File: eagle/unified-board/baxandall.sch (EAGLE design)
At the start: 75 parts, among them IC101 THAT151x, J103 phantom, J104 eqout, J601 micout, U101 OPAMPLME49710, U601 LM3915N, U602 LM3915N, U603 OPAMPLME49710

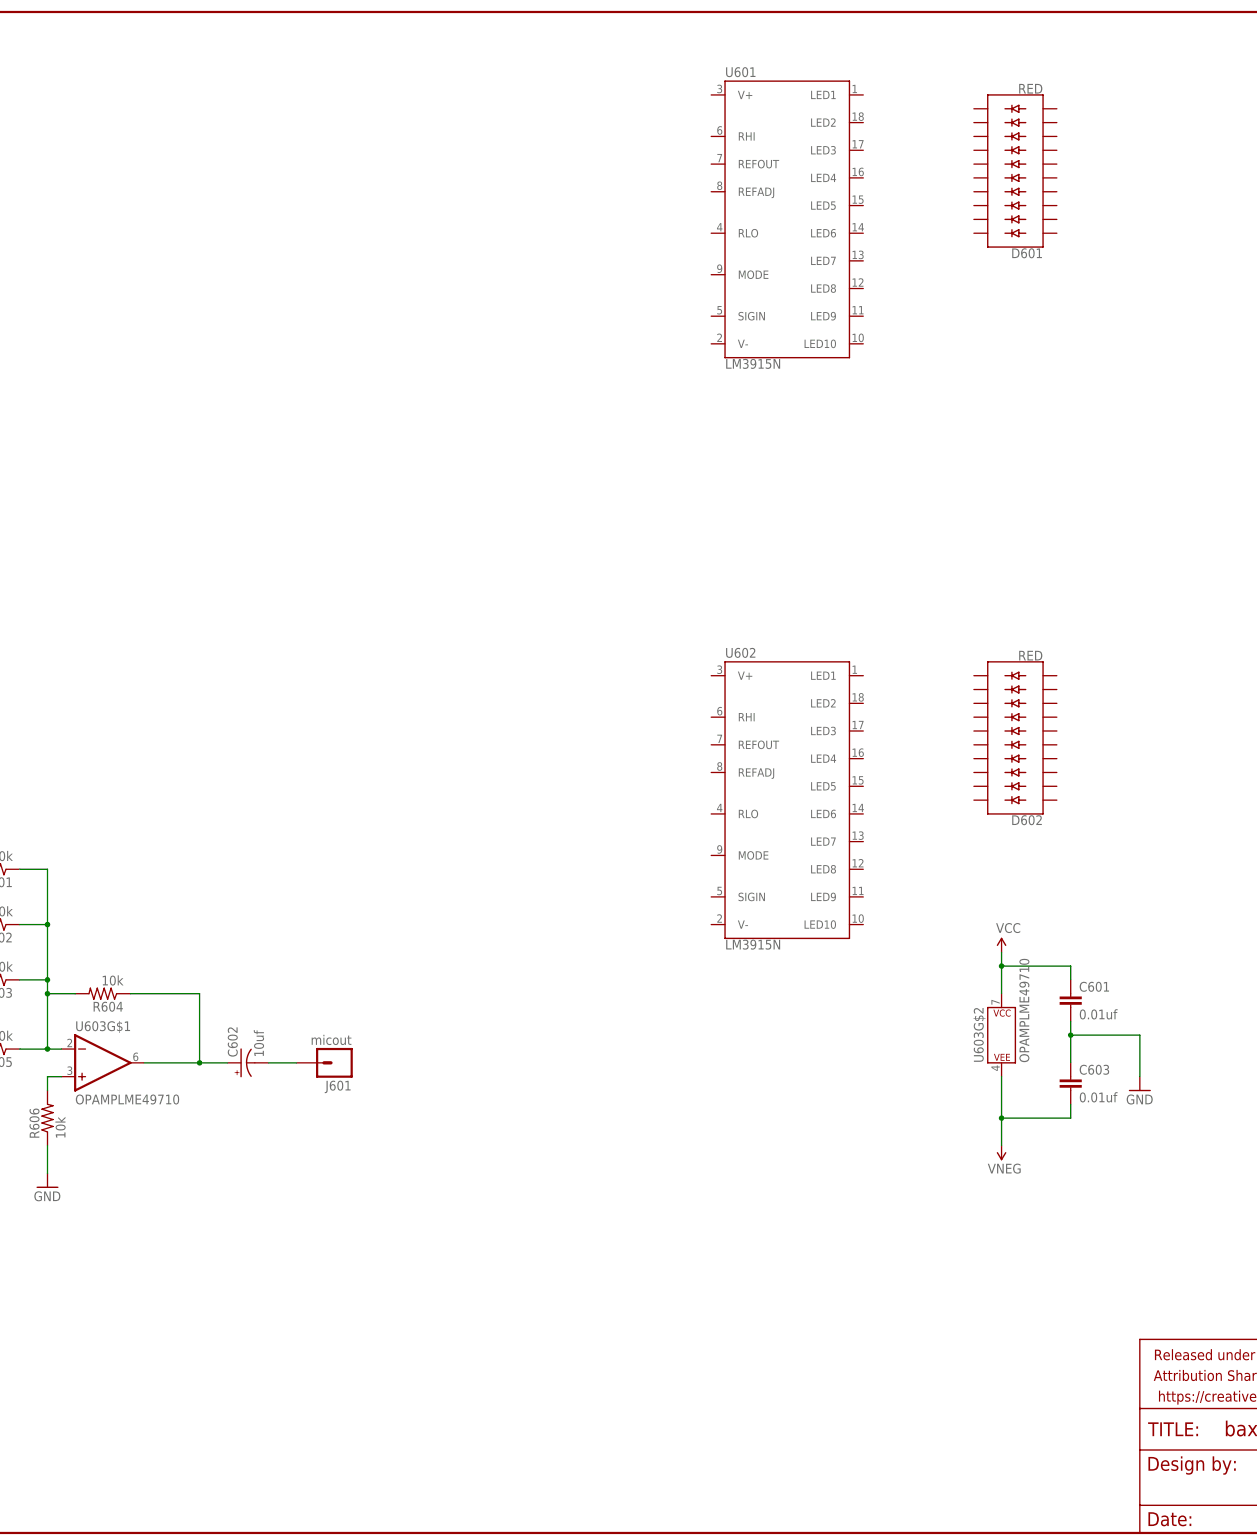
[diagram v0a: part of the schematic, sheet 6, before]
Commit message: A couple more bits done up.
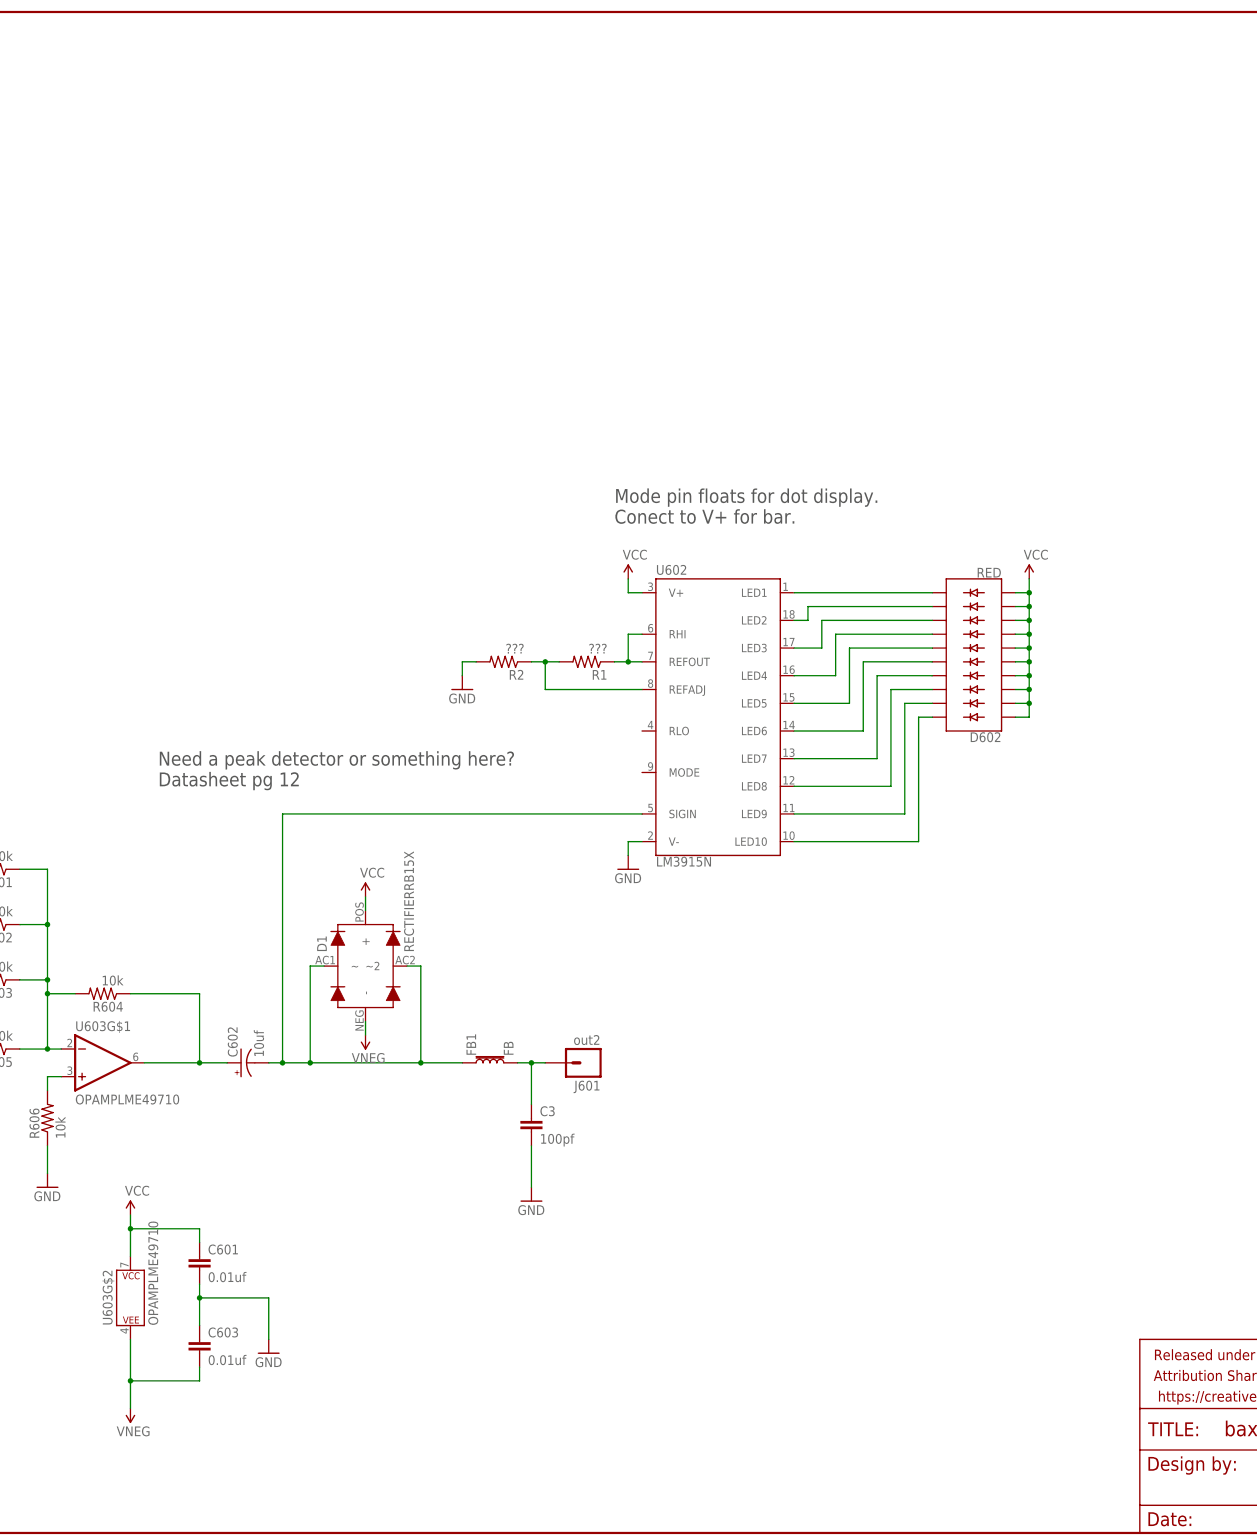
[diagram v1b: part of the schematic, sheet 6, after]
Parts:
- removed D601: RED, SparkFun-LED:LED_BARGRAPH_10RED
- removed U601: LM3915N, SparkFun-IC-Special-Function:LM3915N
- added C3: 100pf, SparkFun-Capacitors:CAPPTH
- added D1: RECTIFIERRB15X, mixer:RECTIFIERRB15X
- added FB1: FB, mixer:FB
- added R1, R2: ???, SparkFun-Resistors:RESISTORAXIAL-0.3
- J601: value micout -> out2
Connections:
- removed net N$18: C602.-, J601.1
- new net N$11: C602.-, D1.~, D1.~2, FB1.1, U602.SIGIN
- new net N$20: D602.C9, U602.LED1
- new net N$41: D602.C8, U602.LED2
- new net N$43: D602.C7, U602.LED3
- new net N$44: D602.C6, U602.LED4
- new net N$45: D602.C5, U602.LED5
- new net N$46: D602.C4, U602.LED6
- new net N$47: D602.C3, U602.LED7
- new net N$48: D602.C2, U602.LED8
- new net N$49: D602.C1, U602.LED9
- new net N$50: D602.C, U602.LED10
- new net N$51: R1.1, U602.REFOUT, U602.RHI
- new net N$52: R1.2, R2.1, U602.REFADJ
- new net N$7: C3.1, FB1.2, J601.1
- net GND: now also C3.2, R2.2, U602.V-
- net VCC: now also D1.+, D602.A, D602.A1, D602.A2, D602.A3, D602.A4, D602.A5, D602.A6, D602.A7, D602.A8, D602.A9, U602.V+
- net VNEG: now also D1.-
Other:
- note added: "Mode pin floats for dot display. Conect to V+ for bar."
- note added: "Need a peak detector or something here? Datasheet pg 12"
- moved on the sheet: C601, C603, D602, J601, U602, U603G$2
